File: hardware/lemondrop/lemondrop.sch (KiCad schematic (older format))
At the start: 80 parts, among them P1 GSG-SMA-CONN, P2 GSG-SMA-CONN, P3 CONN_3X2, P4 CONN_3X2, P5 CONN_20, P6 CONN_8X2, P7 CONN_6X2, P8 GSG-SMA-CONN, P9 CONN_2, T1 BALUN, T2 BALUN, U1 MAX5864, U2 MAX2837, U3 SI5351C, X1 GSG-XTAL4PIN

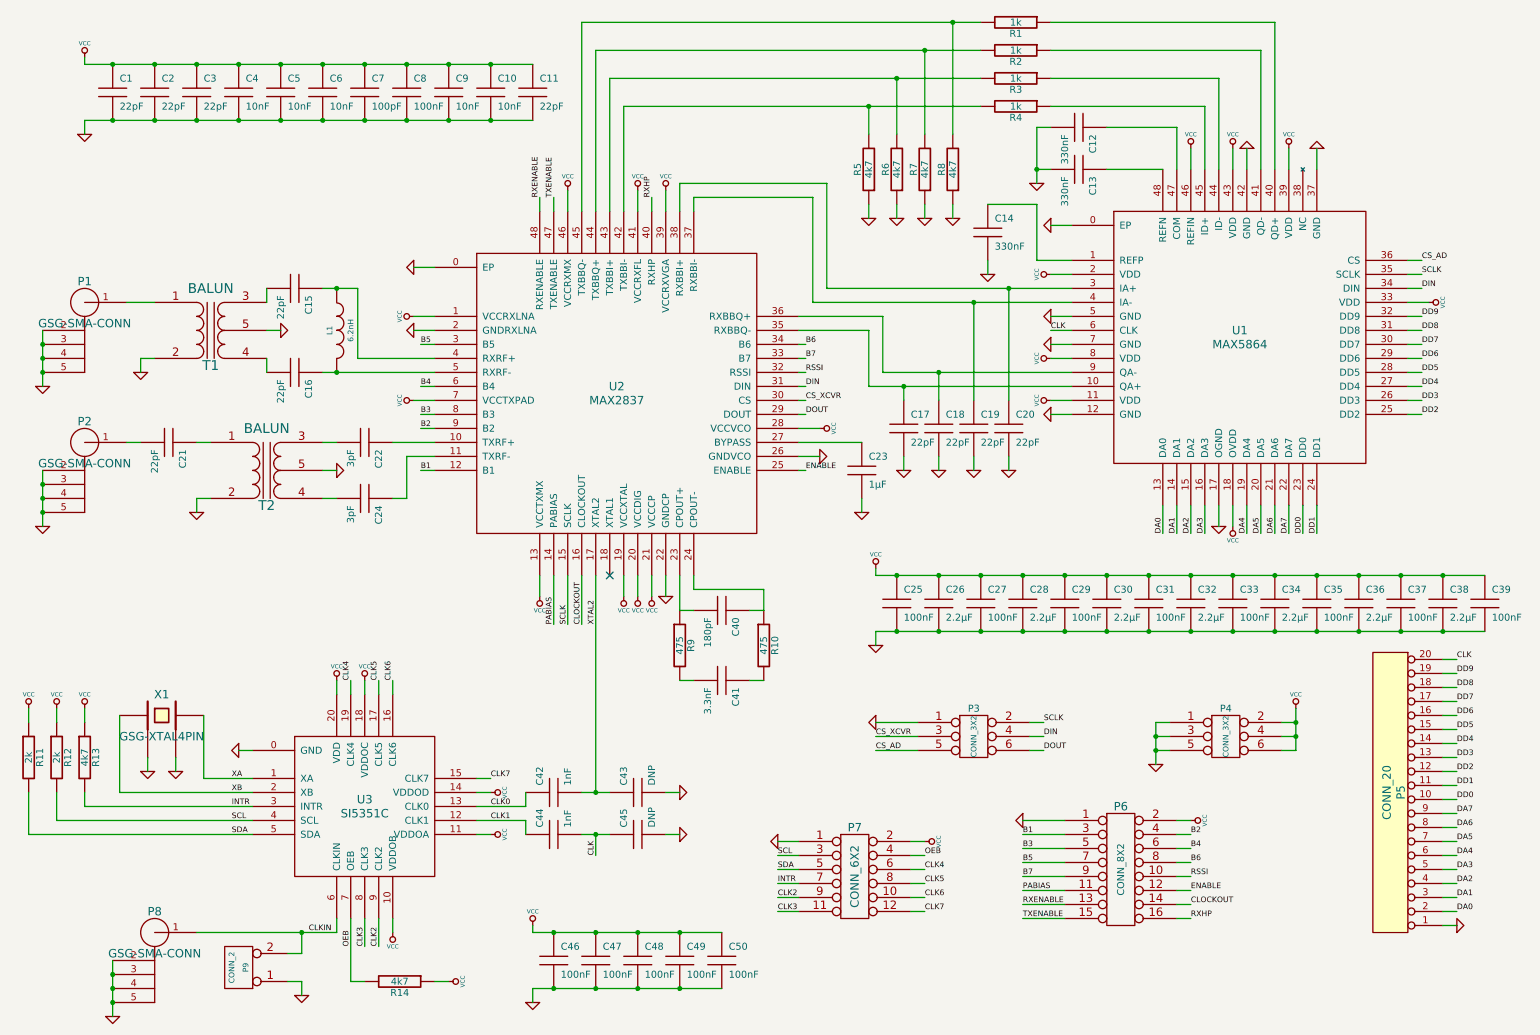
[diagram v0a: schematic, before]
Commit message: various fixes and suggestions from Jared
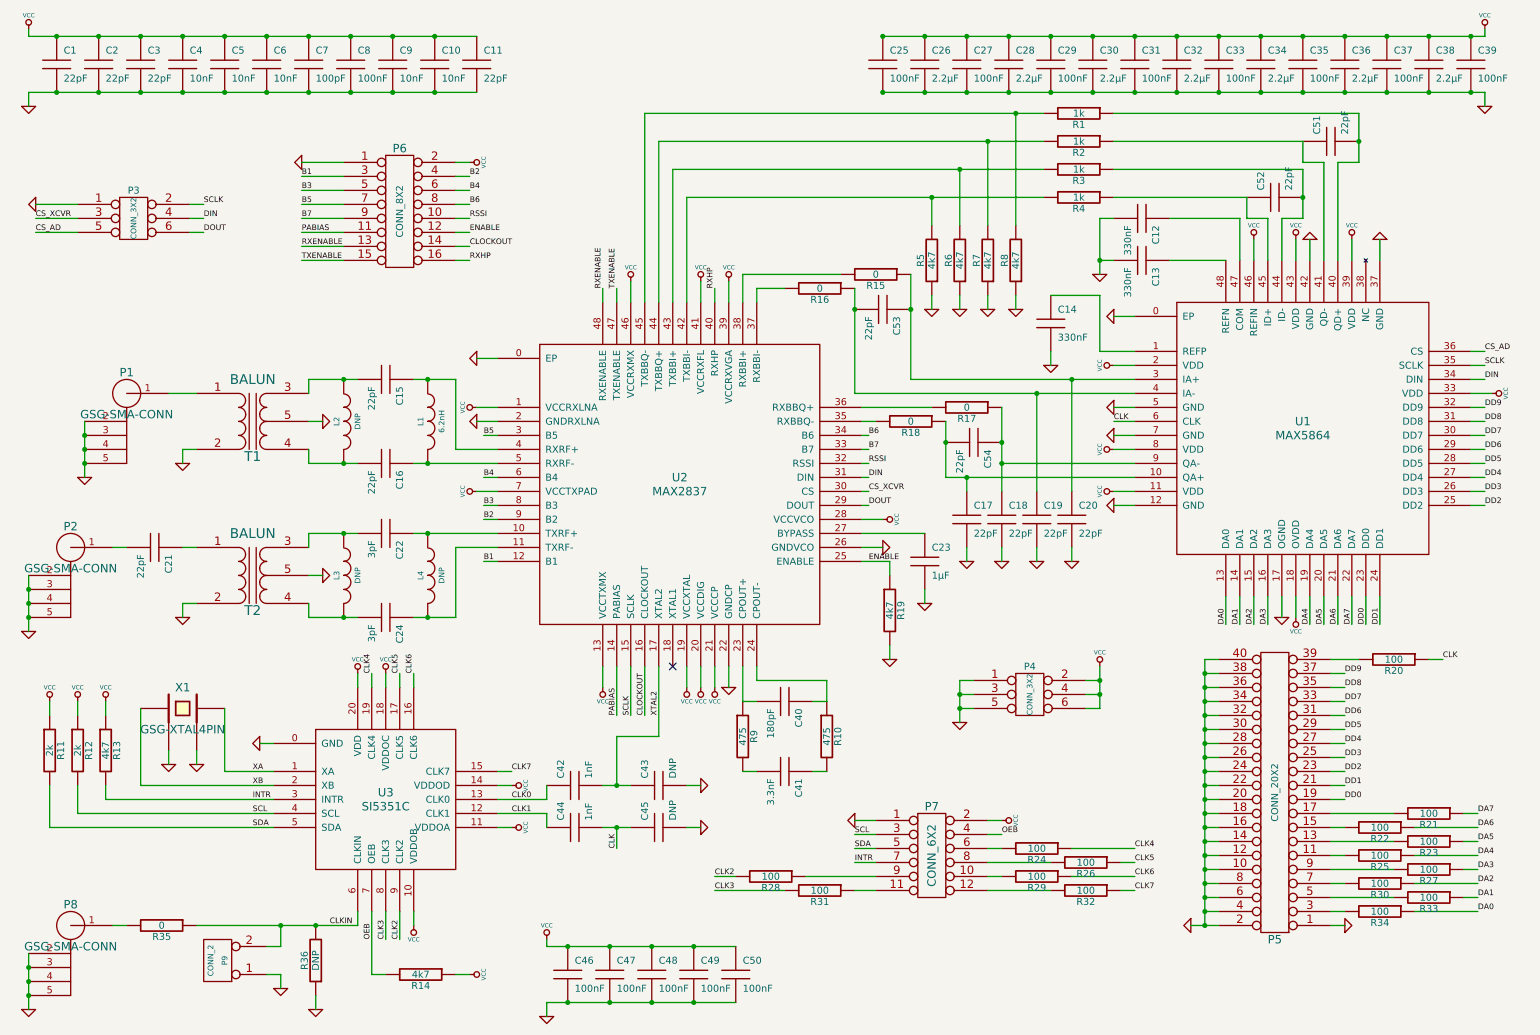
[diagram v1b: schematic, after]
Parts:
- removed P5: CONN_20, symbol CONN_20
- added C51, C52, C53, C54: 22pF, symbol C
- added L2, L3, L4: DNP, symbol INDUCTOR
- added P5: CONN_20X2, symbol CONN_20X2
- added R15, R16, R17, R18, R35: 0, symbol R
- added R19: 4k7, symbol R
- added R20, R21, R22, R23, R24, R25, R26, R27, R28, R29, R30, R31, R32, R33, R34: 100, symbol R
- added R36: DNP, symbol R
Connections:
- net CLK: now also R20.1
- net CLK2: now also R28.2; no longer P7.9
- net CLK3: now also R31.2; no longer P7.11
- net CLK4: now also R24.1; no longer P7.6 (P6)
- net CLK5: now also R26.1; no longer P7.8 (P8)
- net CLK6: now also R29.1; no longer P7.10
- net CLK7: now also R32.1; no longer P7.12
- net CLKIN: now also R35.1, R36.2; no longer P8.1 (RF)
- net DA0: now also R34.1
- net DA1: now also R33.1
- net DA2: now also R30.1
- net DA3: now also R27.1
- net DA4: now also R25.1
- net DA5: now also R23.1
- net DA6: now also R22.1
- net DA7: now also R21.1
- net DD0: now also P5.19 (P19)
- net DD1: now also P5.21 (P21)
- net DD2: now also P5.23 (P23)
- net DD3: now also P5.25
- net DD4: now also P5.27 (P27)
- net DD5: now also P5.29 (P29)
- net DD6: now also P5.31 (P31)
- net DD7: now also P5.33 (P33)
- net DD8: now also P5.35 (P35)
- net DD9: now also P5.37 (P37)
- net ENABLE: now also R19.1
- net GND: now also P5.1 (P1), P5.10 (P10), P5.12 (P12), P5.14 (P14), P5.16 (P16), P5.18 (P18), P5.2 (P2), P5.20 (P20), P5.22 (P22), P5.24 (P24), P5.26 (P26), P5.28 (P28), P5.30 (P30), P5.32 (P32), P5.34 (P34), P5.36 (P36), P5.38 (P38), P5.4 (P4), P5.40 (P40), P5.6 (P6), P5.8 (P8), R19.2, R36.1
- net at C22.1, U2.10 (TXRF+): now also L4.1
- net at C24.1, U2.11 (TXRF-): now also L4.2
- net at C17.1, U1.10 (QA+): now also C54.2, R18.1; no longer U2.35 (RXBBQ-)
- net at C18.1, U1.9 (QA-): now also C54.1, R17.1; no longer U2.36 (RXBBQ+)
- net at C19.1, U1.4 (IA-): now also C53.2, R16.1; no longer U2.37 (RXBBI-)
- net at C20.1, U1.3 (IA+): now also C53.1, R15.1; no longer U2.38 (RXBBI+)
- net at R1.1, U1.40 (QD+): now also C51.2
- net at R2.1, U1.41 (QD-): now also C51.1
- net at R3.1, U1.44 (ID-): now also C52.2
- net at R4.1, U1.45 (ID+): now also C52.1
- net at C15.2, T1.3 (PR2): now also L2.1
- net at C16.2, T1.4 (PR1): now also L2.2
- net at C24.2, T2.4 (PR1): now also L3.2
- net at C22.2, T2.3 (PR2): now also L3.1
- new net: R18.2, U2.35 (RXBBQ-)
- new net: R17.2, U2.36 (RXBBQ+)
- new net: R16.2, U2.37 (RXBBI-)
- new net: R15.2, U2.38 (RXBBI+)
- new net: P8.1 (RF), R35.2
- new net: P7.10, R29.2
- new net: P7.11, R31.1
- new net: P7.12, R32.2
- new net: P7.6 (P6), R24.2
- new net: P7.8 (P8), R26.2
- new net: P7.9, R28.1
- new net: P5.11 (P11), R25.2
- new net: P5.13 (P13), R23.2
- new net: P5.15 (P15), R22.2
- new net: P5.17 (P17), R21.2
- new net: P5.3 (P3), R34.2
- new net: P5.39 (P39), R20.2
- new net: P5.5 (P5), R33.2
- new net: P5.7 (P7), R30.2
- new net: P5.9 (P9), R27.2
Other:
- moved on the sheet: C1, C10, C11, C12, C13, C14, C15, C16, C17, C18, C19, C2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
